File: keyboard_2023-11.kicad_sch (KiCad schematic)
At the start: 80 parts, among them J1 Conn_01x04, J11 Conn_01x07_Socket, J2 Conn_01x04_Socket, J3 Conn_01x07_Socket, J4 Conn_01x07_Pin, J5 Conn_01x04_Socket, J6 Conn_01x07_Pin, J7 Conn_01x04_Socket, SW1 SW_Push, SW10 SW_Push, SW11 SW_Push, SW12 SW_Push, SW13 SW_Push, SW14 SW_Push, SW15 SW_Push, SW16 SW_Push, SW17 SW_Push, SW18 SW_Push, SW19 SW_Push, SW2 SW_Push, SW20 SW_Push, SW21 SW_Push, SW22 SW_Push, SW23 SW_Push, SW24 SW_Push, SW3 SW_Push, SW4 SW_Push, SW5 SW_Push, SW6 SW_Push, SW7 SW_Push, SW8 SW_Push, SW9 SW_Push, U1 MCP23017_SO, U2 MCP23017_SO

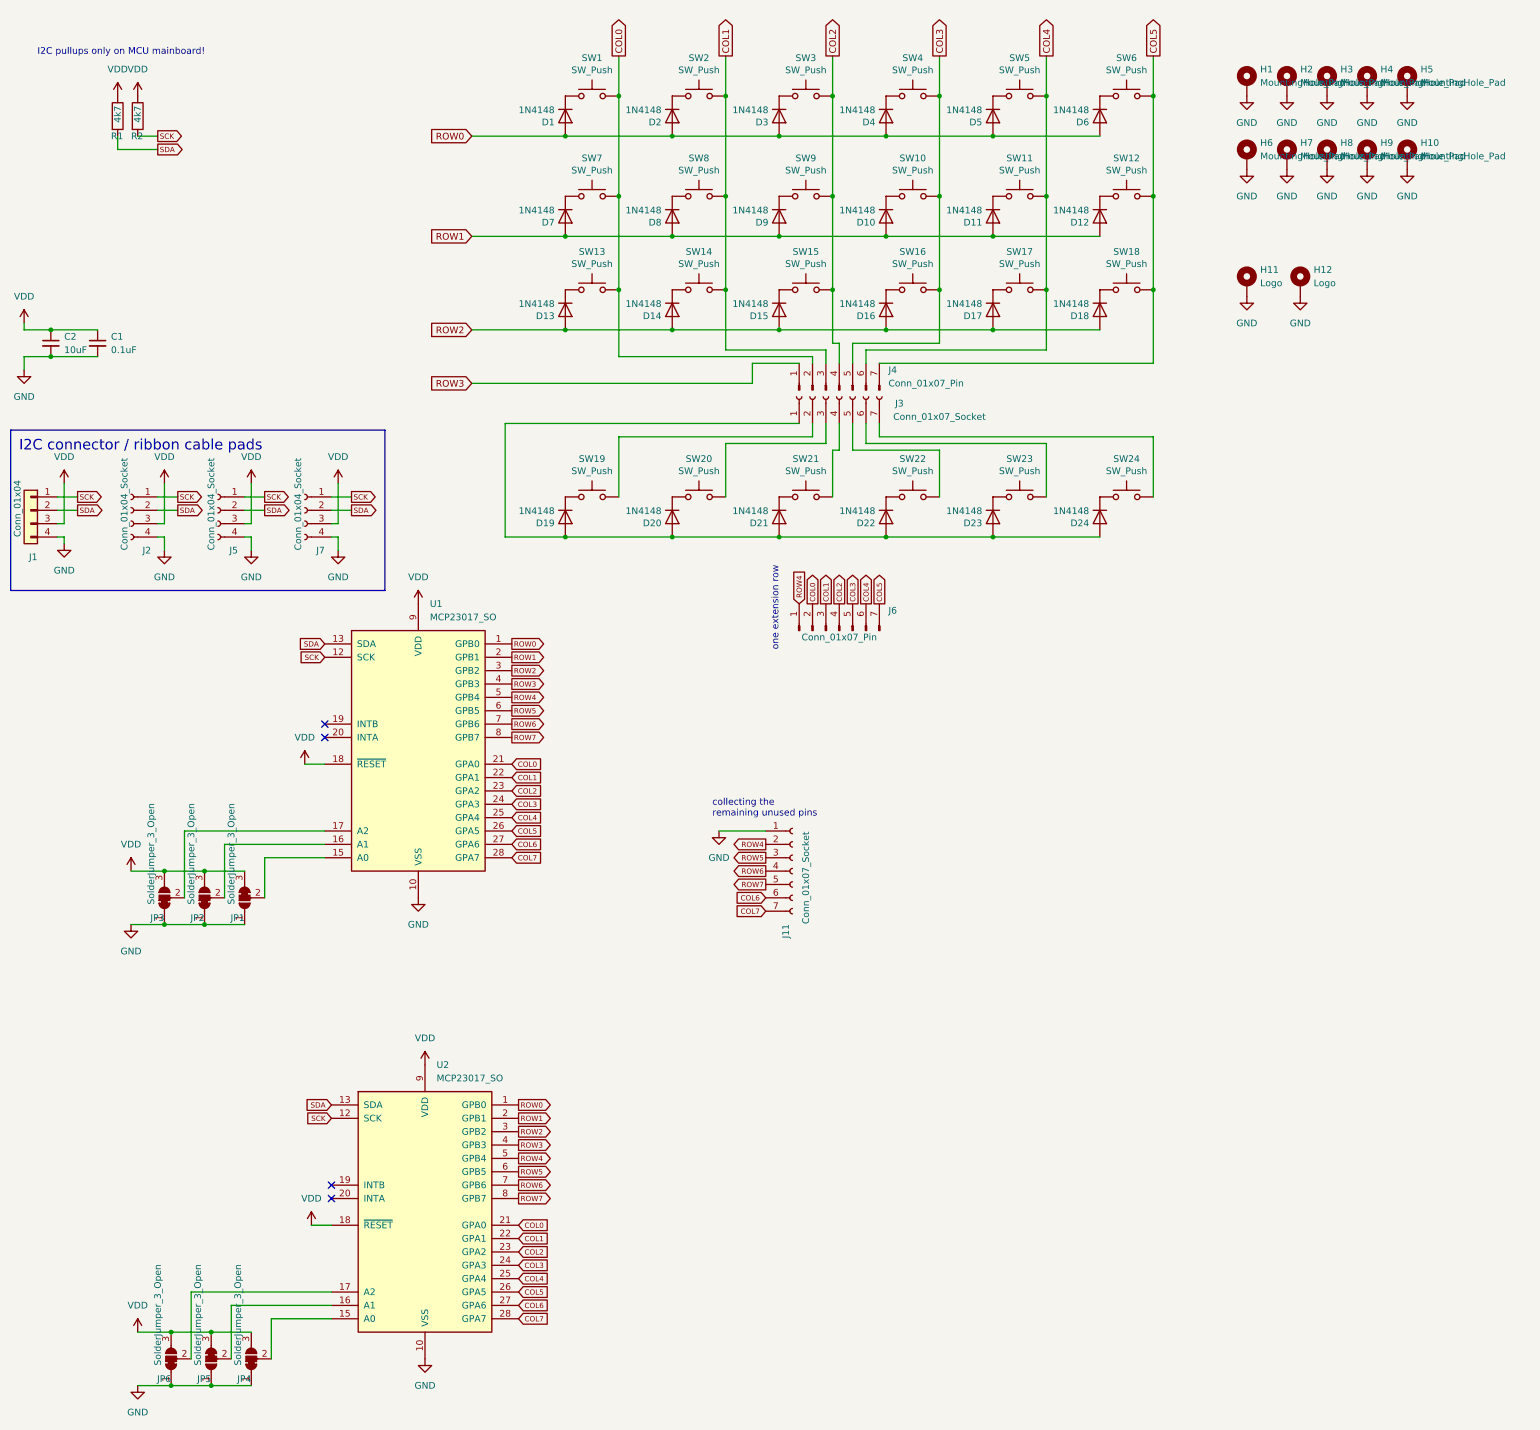
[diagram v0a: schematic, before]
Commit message: cleanup schematic for release
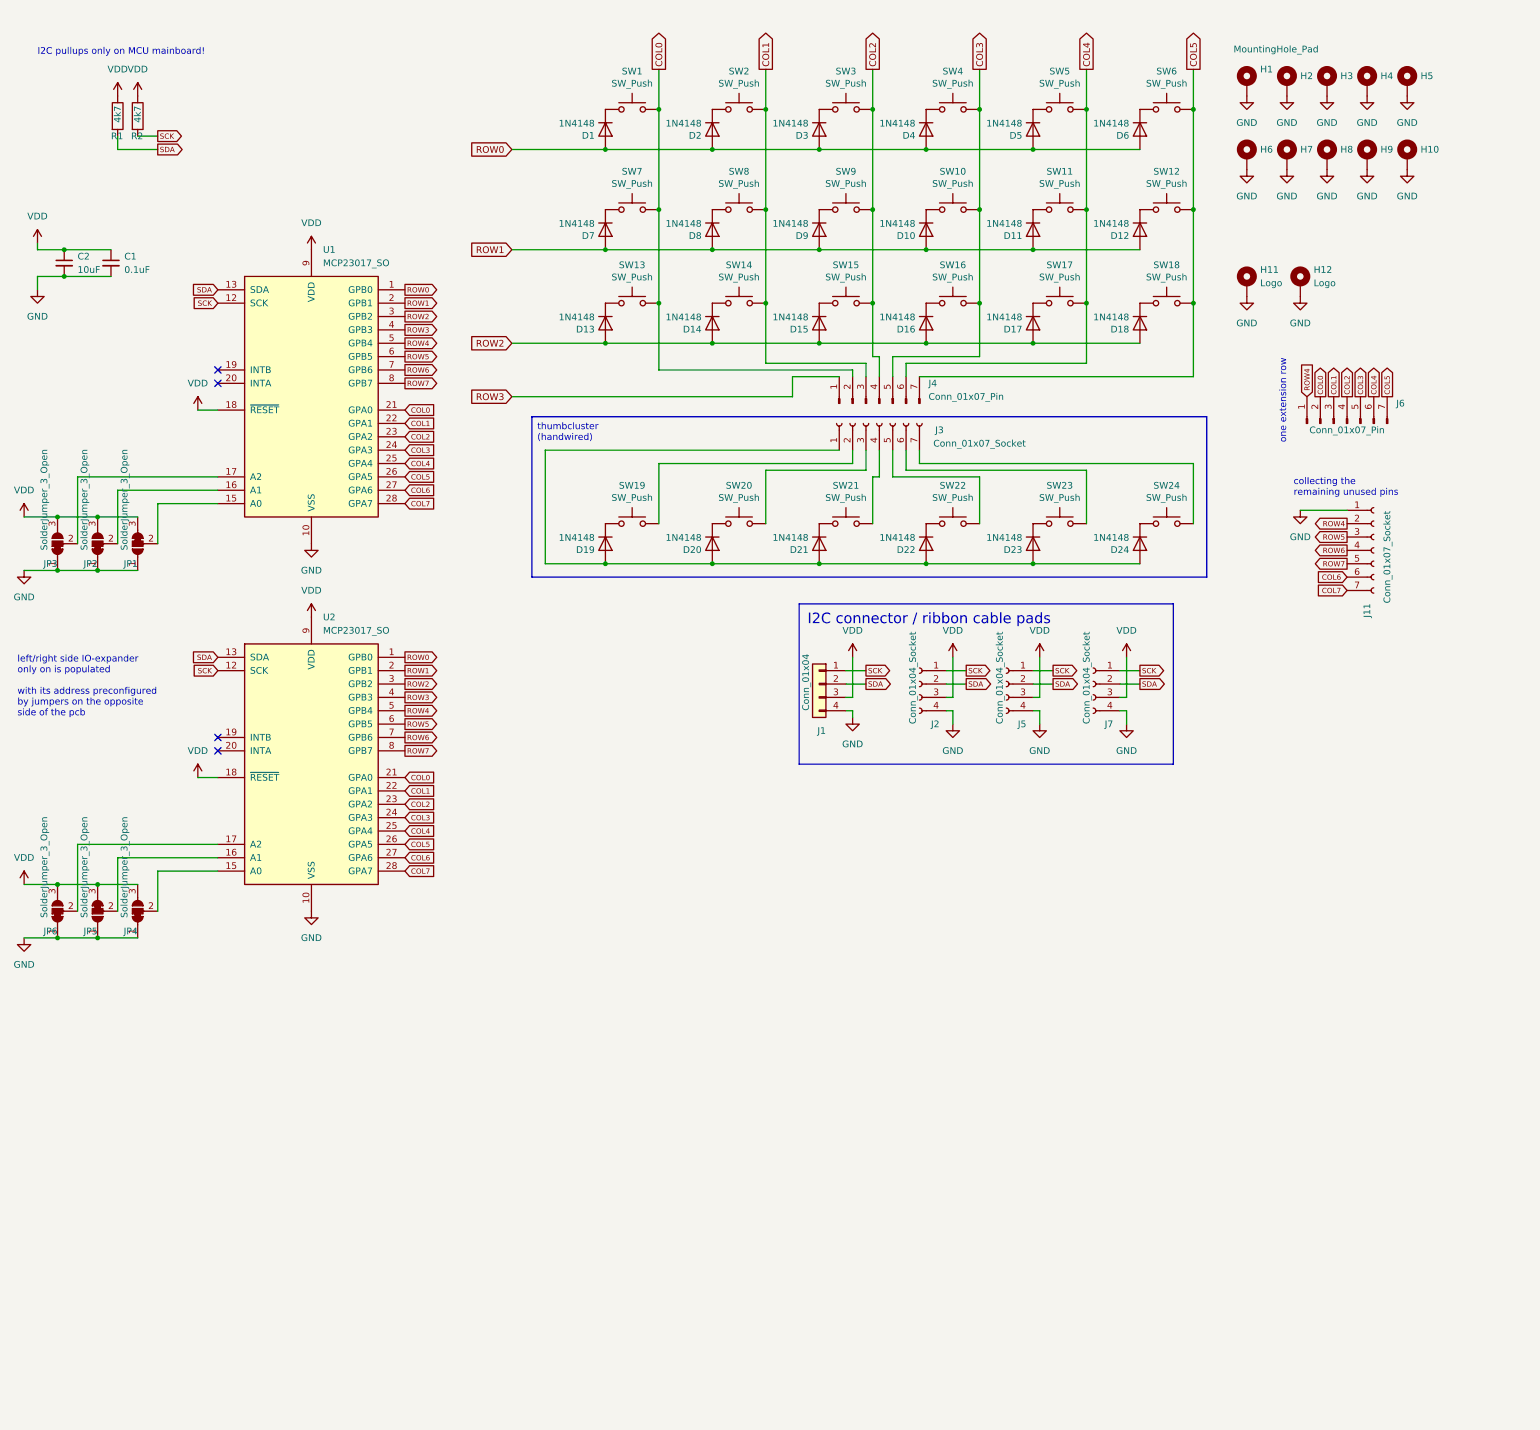
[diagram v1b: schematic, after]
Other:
- note added: "left/right side IO-expander only on is populated with its address preconfigured by jumpers on the opposite side of the pcb"
- moved on the sheet: C1, C2, D1, D10, D11, D12, D13, D14, D15, D16, D17, D18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
